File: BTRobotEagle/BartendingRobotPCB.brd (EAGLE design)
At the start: 154.9 x 100 mm, 32 parts, among them P1 B2B-XH-A(LF)(SN), P10 B2B-XH-A(LF)(SN), P11 B2B-XH-A(LF)(SN), P2 B2B-XH-A(LF)(SN), P3 B2B-XH-A(LF)(SN), P4 B2B-XH-A(LF)(SN), P5 B2B-XH-A(LF)(SN), P6 B2B-XH-A(LF)(SN), P7 B2B-XH-A(LF)(SN), P8 B2B-XH-A(LF)(SN), P9 B2B-XH-A(LF)(SN), U10 MCP23017-E/SP, U11 MCP23017-E/SP

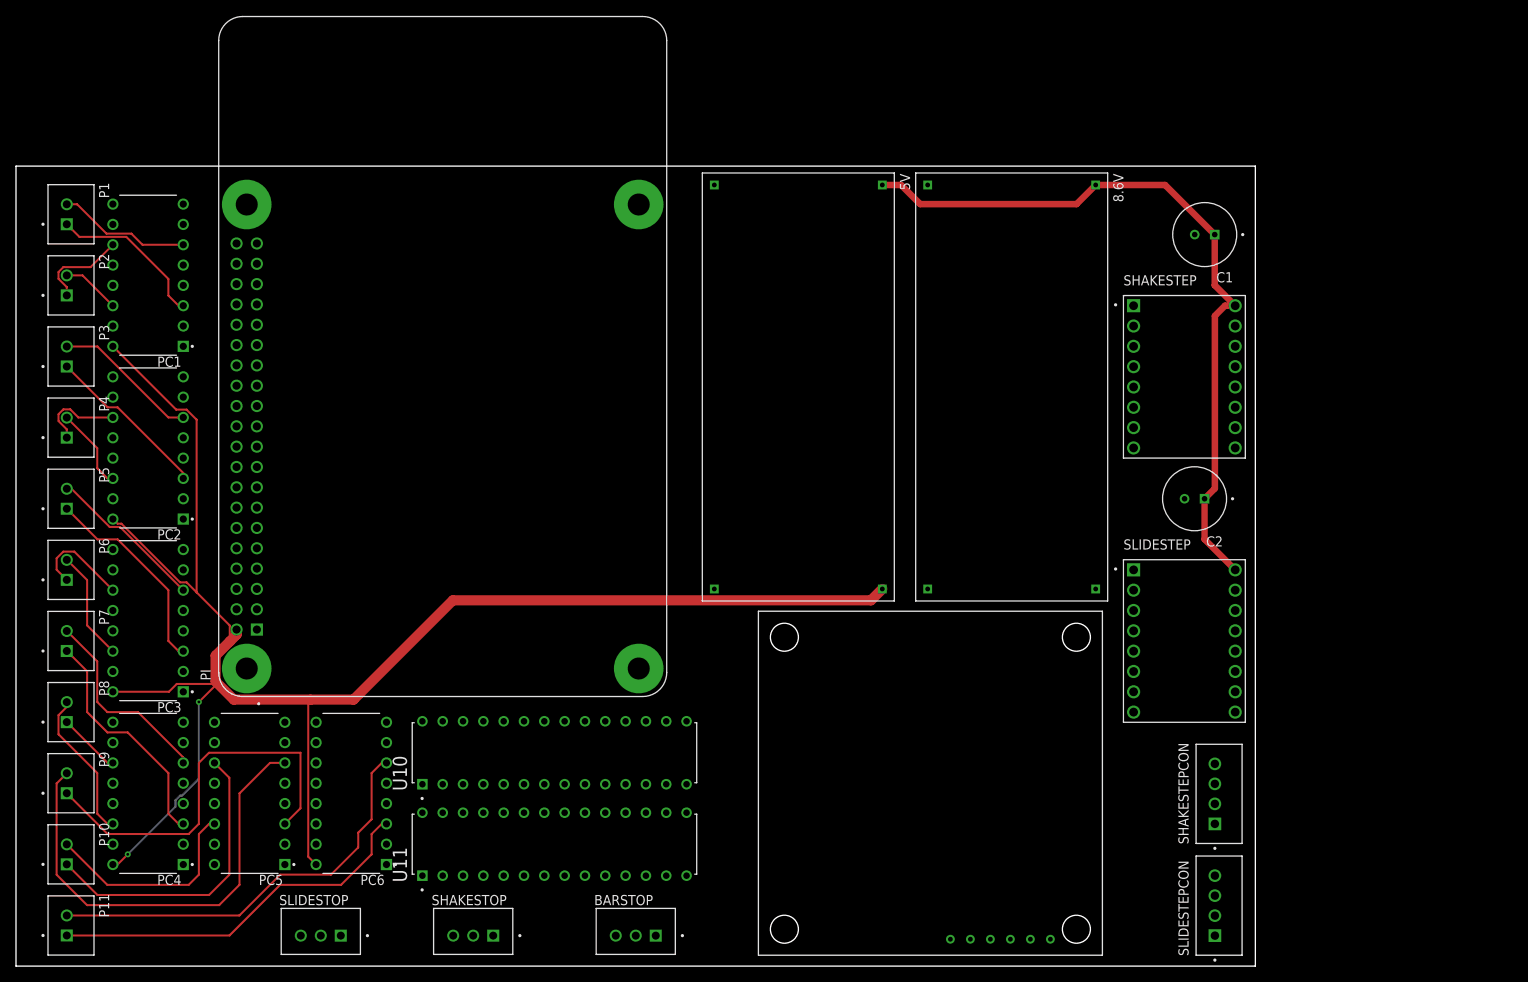
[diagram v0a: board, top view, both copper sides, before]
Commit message: BRD/SCH upgrades
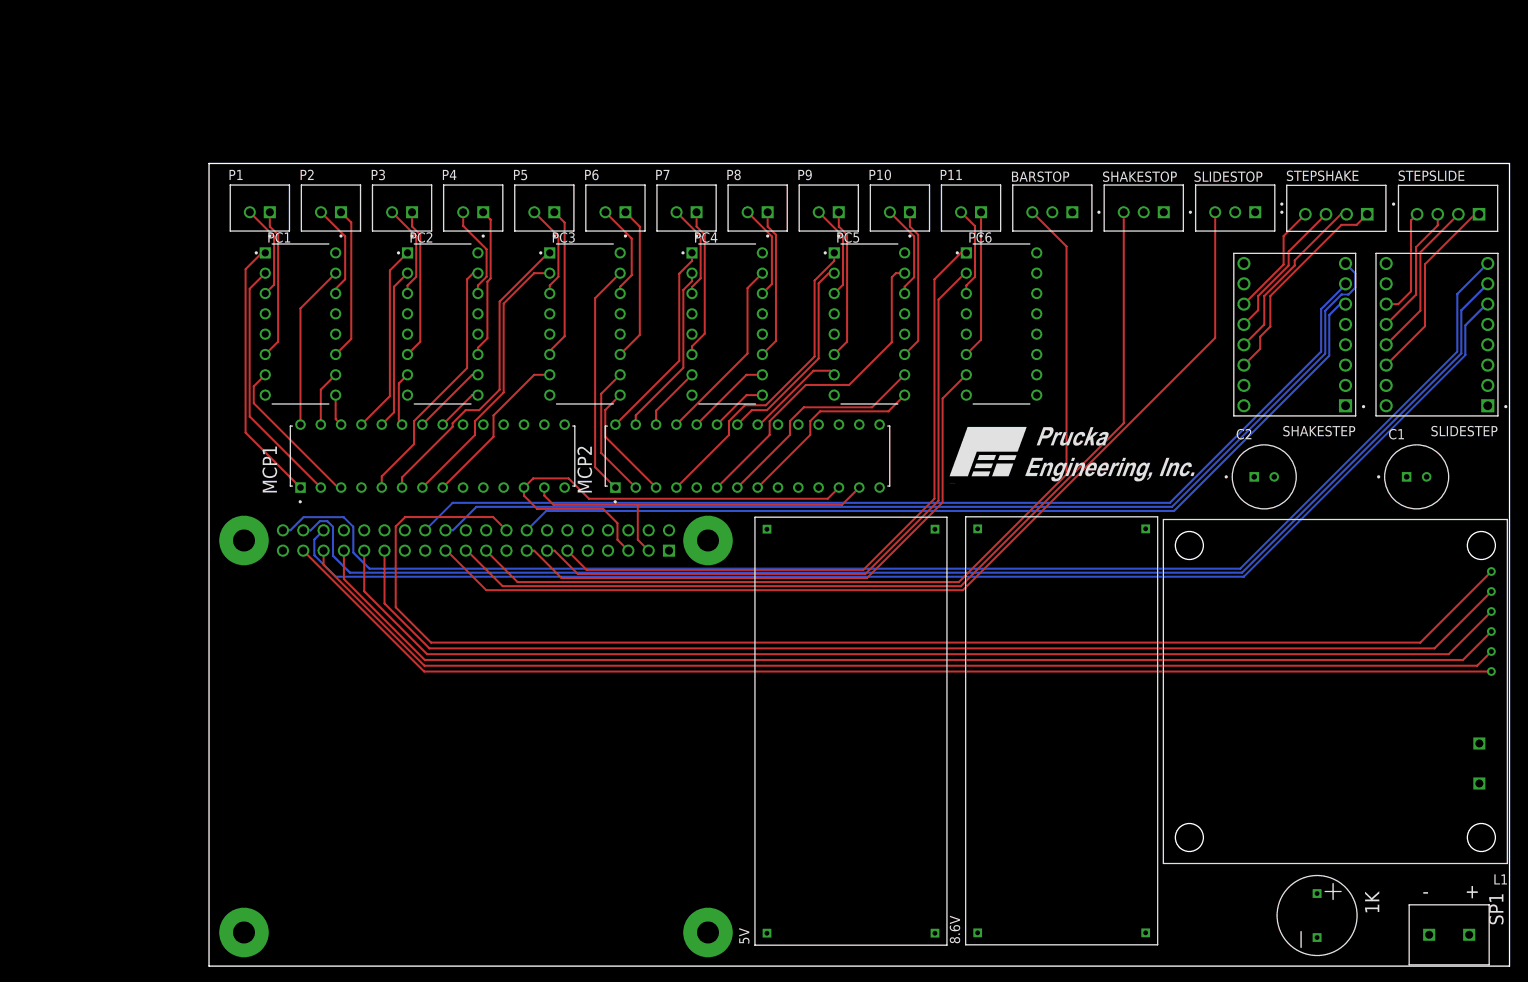
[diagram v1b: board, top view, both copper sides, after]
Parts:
- removed 12VMOTORS: L298N, BartendingRobot:L298N
- removed SHAKESTEPCON, SLIDESTEPCON: B4B-XH-A(LF)(SN), BartendingRobot:JST_B4B-XH-A(LF)(SN)
- removed U10, U11: MCP23017-E/SP, BartendingRobot:DIP787W45P254L3556H508Q28
- added 1K: 10MMCAP, BartendingRobot:10MMCAP
- added L1: L298N, BartendingRobot:L298N
- added MCP1, MCP2: MCP23017-E/SP, BartendingRobot:DIP787W45P254L3556H508Q28
- added SP1: 2PORTSCREW, BartendingRobot:2PORTSCREW
- added STEPSHAKE, STEPSLIDE: B4B-XH-A(LF)(SN), BartendingRobot:JST_B4B-XH-A(LF)(SN)
- moved SLIDESTOP 145.7 mm to (128.3, 94.2)
- moved P11 144.0 mm to (95.2, 94.2), turned to 0 degrees
- moved P10 131.5 mm to (86.4, 94.2), turned to 0 degrees
- moved SHAKESTOP 123.3 mm to (116.8, 94.2)
- moved P9 119.0 mm to (77.5, 94.2), turned to 0 degrees
- moved P8 106.6 mm to (68.6, 94.2), turned to 0 degrees
- moved BARSTOP 104.3 mm to (105.4, 94.2)
- moved PC6 100.2 mm to (99.1, 80.3), turned to 0 degrees
- moved PC5 97.2 mm to (82.5, 80.3), turned to 0 degrees
- moved P7 94.2 mm to (59.7, 94.2), turned to 0 degrees
- moved PC4 93.2 mm to (64.8, 80.3), turned to 0 degrees
- moved P6 81.9 mm to (50.8, 94.2), turned to 0 degrees
- moved P5 69.6 mm to (41.9, 94.2), turned to 0 degrees
- moved PC3 66.0 mm to (47.0, 80.3), turned to 0 degrees
- moved P4 57.5 mm to (33.0, 94.2), turned to 0 degrees
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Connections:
- removed net N$31: P9.2, PC5.6
- removed net N$32: P9.1, PC5.3
- removed net N$35: P7.2, PC4.6
- removed net N$36: P7.1, PC4.3
- removed net SHIELD: PI.S1, PI.S2, PI.S3, PI.S4
- new net N$10: P3.2, PC2.3
- new net N$20: P11.2, PC6.3
- new net N$25: P1.1, PC1.6
- new net N$9: P3.1, PC2.6
- net 0: now also MCP1.1; no longer U11.21
- net 1: now also MCP1.2; no longer U11.22
- net 10: now also MCP1.22; no longer U11.3
- net 11: now also MCP1.5; no longer U11.4
- net 12: now also MCP1.6; no longer U11.5
- net 12V: now also 1K.+, L1.12V, SP1.P1
- net 13: now also MCP1.7; no longer U11.6
- net 14: now also MCP1.8; no longer U11.7
- net 15: now also MCP2.3; no longer U10.21
- net 16: now also MCP2.2; no longer U10.22
- net 17: now also MCP2.1; no longer U10.23
- net 18: now also MCP2.28; no longer U10.24
- net 19: now also MCP2.27; no longer U10.25
- net 2: now also MCP1.3; no longer U11.23
- net 20: now also MCP2.26; no longer U10.26
- net 21: now also MCP2.23; no longer U10.27
- net 22: now also MCP2.24; no longer U10.28
- net 23: now also MCP2.25; no longer U10.1
- net 24: now also MCP2.4; no longer U10.2
- net 25: now also MCP2.22; no longer U10.3
- net 26: now also MCP2.21; no longer U10.4
- net 27: now also MCP2.8; no longer U10.5
- net 28: now also MCP2.7; no longer U10.6
- net 29: now also MCP2.6; no longer U10.7
- net 3: now also MCP1.26; no longer U11.24
- net 3.3V: now also MCP1.18, MCP1.9, MCP2.15, MCP2.18, MCP2.9; no longer BARSTOP.1, SHAKESTOP.1, SLIDESTOP.1, U10.15, U10.18, U10.9, U11.18, U11.9
- net 4: now also MCP1.27; no longer U11.25
- net 5: now also MCP1.28; no longer U11.26
- net 5V: now also BARSTOP.1, SHAKESTOP.1, SLIDESTOP.1
- net 6: now also MCP1.25; no longer U11.27
- net 7: now also MCP1.24; no longer U11.28
- net 8: now also MCP1.23; no longer U11.1
- net 9: now also MCP1.21; no longer U11.2
- net BARST: now also PI.19; no longer PI.21
- net CGND: now also 1K.-, L1.GND, MCP1.10, MCP1.15, MCP1.16, MCP1.17, MCP2.10, MCP2.16, MCP2.17, PI.S1, PI.S2, PI.S3, PI.S4, SP1.P2; no longer U10.10, U10.16, U10.17, U11.10, U11.15, U11.16, U11.17
- net ICE1: now also L1.IN4; no longer 12VMOTORS.IN1
- net ICE2: now also L1.IN3; no longer 12VMOTORS.IN2
- net ICEEN: now also L1.ENB; no longer 12VMOTORS.ENA
- net N$1: now also SHAKESTEP.14, STEPSHAKE.1; no longer SHAKESTEP.12, SHAKESTEPCON.4
- net N$11: now also P7.1, PC4.6; no longer P1.1, PC1.3
- net N$12: now also P7.2, PC4.3; no longer P1.2, PC1.6
- net N$15: now also P9.1, PC5.6; no longer P3.1, PC2.3
- net N$16: now also P9.2, PC5.3; no longer P3.2, PC2.6
- net N$19: now also P11.1, PC6.6; no longer P5.1, PC3.3
- net N$2: now also SHAKESTEP.13, STEPSHAKE.2; no longer SHAKESTEP.11, SHAKESTEPCON.3
- net N$21: now also P5.1; no longer P5.2
- net N$24: now also P5.2, PC3.3; no longer P11.1, PC6.3
- net N$26: now also P1.2, PC1.3; no longer P11.2, PC6.6
- net N$3: now also SHAKESTEP.11, STEPSHAKE.4; no longer SHAKESTEP.13, SHAKESTEPCON.2
- net N$4: now also SHAKESTEP.12, STEPSHAKE.3; no longer SHAKESTEP.14, SHAKESTEPCON.1
- net N$5: now also SLIDESTEP.14, STEPSLIDE.1; no longer SLIDESTEP.12, SLIDESTEPCON.4
- net N$6: now also SLIDESTEP.13, STEPSLIDE.2; no longer SLIDESTEP.11, SLIDESTEPCON.3
- net N$7: now also SLIDESTEP.11, STEPSLIDE.4; no longer SLIDESTEP.13, SLIDESTEPCON.2
- net N$8: now also SLIDESTEP.12, STEPSLIDE.3; no longer SLIDESTEP.14, SLIDESTEPCON.1
- net SCL: now also MCP1.12, MCP2.12; no longer U10.12, U11.12
- net SDA: now also MCP1.13, MCP2.13; no longer U10.13, U11.13
- net SHAKE1: now also L1.IN1; no longer 12VMOTORS.IN3
- net SHAKE2: now also L1.IN2; no longer 12VMOTORS.IN4
- net SHAKEEN: now also L1.ENA; no longer 12VMOTORS.ENB
- net SHAKEST: now also PI.21; no longer PI.19
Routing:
- net 5V: track 218.8 -> 0.00 mm, vias 2 -> 0
- net SLIDEDIR: track 0.00 -> 175.9 mm
- net SLIDESTEP: track 0.00 -> 171.4 mm
- net SLIDESLP: track 0.00 -> 167.7 mm
- net ICEEN: track 0.00 -> 167.6 mm
- net SHAKEEN: track 0.00 -> 154.8 mm
- net SHAKE1: track 0.00 -> 153.7 mm
- net SHAKE2: track 0.00 -> 152.6 mm
- net ICE2: track 0.00 -> 151.4 mm
- net ICE1: track 0.00 -> 150.2 mm
- net SHAKEDIR: track 0.00 -> 132.9 mm
- net SHAKESTEP: track 0.00 -> 131.0 mm
- net SLIDEST: track 0.00 -> 127.0 mm
- net SHAKEST: track 0.00 -> 118.9 mm
- net SHAKESLP: track 0.00 -> 117.0 mm
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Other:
- board size 154.9 x 100 mm -> 162.6 x 100.3 mm
- board text added: "C:/Temp/PEI Logo.bmp"
